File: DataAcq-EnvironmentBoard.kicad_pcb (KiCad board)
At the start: 2 copper layers, 73.5 x 63.2 mm, 13 parts, among them J1 CAN Output, J2 CAN Input, U1 SHT45, U2 FS3000-1005, U3 LMT87DCK, U4 Daughterboard Connector

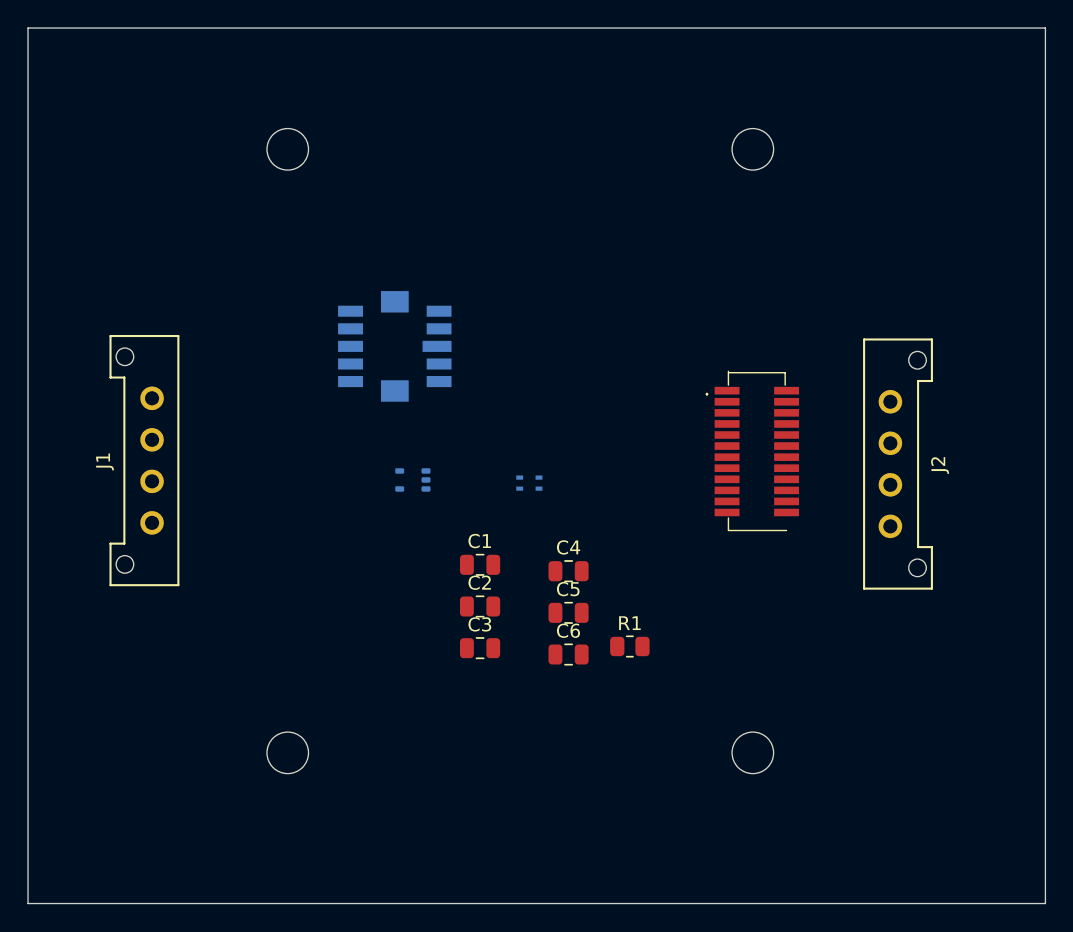
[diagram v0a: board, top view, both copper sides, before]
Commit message: initial layout/routing
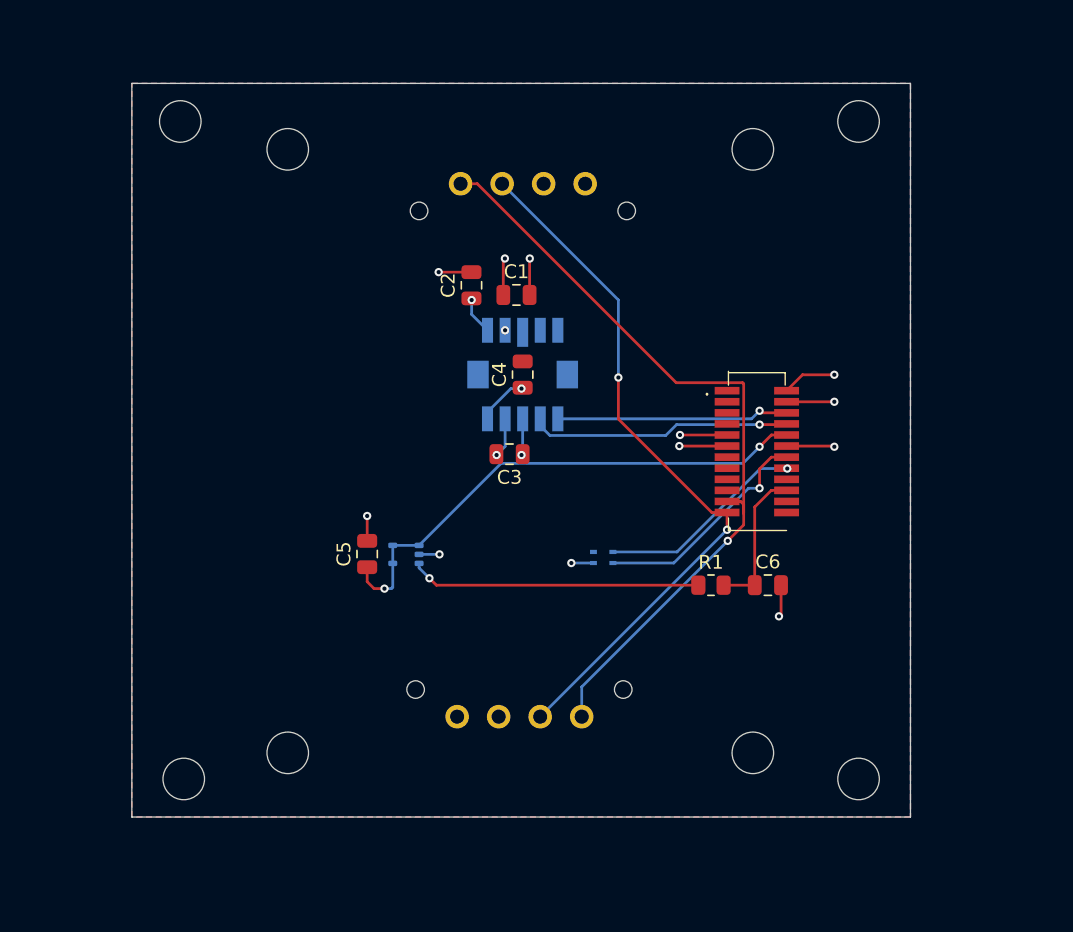
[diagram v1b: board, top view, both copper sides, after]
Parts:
- added MH1: M.3, MountingHole:MountingHole_3mm, F.Cu at (136.8, 72.5)
- added MH2: M.3, MountingHole:MountingHole_3mm, F.Cu at (137.0, 120.0)
- added MH3: M.3, MountingHole:MountingHole_3mm, F.Cu at (185.8, 72.5)
- added MH4: M.3, MountingHole:MountingHole_3mm, F.Cu at (185.8, 120.0)
- J1, J2: moved to B.Cu
- moved J2 34.8 mm to (157.0, 77.0), turned to 0 degrees
- moved J1 34.1 mm to (165.8, 115.5), turned to 180 degrees
- moved C2 23.2 mm to (157.8, 84.3), turned to 90 degrees
- moved C1 19.7 mm to (161.0, 85.0)
- moved C6 15.2 mm to (179.2, 106.0)
- moved C5 15.2 mm to (150.2, 103.8), turned to 90 degrees
- moved C4 14.6 mm to (161.5, 90.8), turned to 90 degrees
- moved C3 14.2 mm to (160.5, 96.5), turned to 180 degrees
- moved U2 9.46 mm to (161.5, 90.8), turned to -90 degrees
- moved U1 7.57 mm to (167.3, 104.0)
- moved R1 7.34 mm to (175.1, 106.0)
- moved U3 5.40 mm to (153.1, 103.8)
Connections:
- net Net-(U2-TP1) renamed /AFLW_TP1
- net Net-(U2-TP2) renamed /AFLW_TP2
- net Net-(U2-VCM) renamed /AFLW_VCM
- net Net-(U2-VREG) renamed /AFLW_VREG
- net Net-(U3-OUT) renamed /TEMP_OUT
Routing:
- net /CAN_L: track 0.00 -> 57.2 mm, vias 0 -> 1
- net /CAN_H: track 0.00 -> 51.5 mm, vias 0 -> 2
- net VDDA: track 0.00 -> 37.9 mm, vias 0 -> 2
- net /TEMP_OUT: track 0.00 -> 21.0 mm, vias 0 -> 1
- net /I2C2_SCL: track 0.00 -> 18.9 mm, vias 0 -> 1
- net /I2C2_SDA: track 0.00 -> 16.8 mm, vias 0 -> 1
- net /I2C1_SCL: track 0.00 -> 16.5 mm, vias 0 -> 1
- net /I2C1_SDA: track 0.00 -> 15.1 mm, vias 0 -> 1
- net GND: track 0.00 -> 11.9 mm, vias 0 -> 4
- net +3.3V: track 0.00 -> 11.6 mm, vias 0 -> 5
- net /PA1(ADC): track 0.00 -> 10.7 mm
- net GNDA: track 0.00 -> 9.06 mm, vias 0 -> 4
- net /AFLW_VCM: track 0.00 -> 3.65 mm, vias 0 -> 1
- net /AFLW_TP2: track 0.00 -> 2.87 mm, vias 0 -> 1
- net /AFLW_VREG: track 0.00 -> 2.66 mm, vias 0 -> 1
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- added copper zone on In2.Cu, net +3.3V
- added copper zone on F.Cu, net /+12V_In
- added copper zone on B.Cu, net GND
- added copper zone on In1.Cu, net GNDA
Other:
- board size 73.5 x 63.2 mm -> 56.2 x 53 mm
- copper layers 2 -> 4
